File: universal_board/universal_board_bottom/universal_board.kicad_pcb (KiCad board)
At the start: 2 copper layers, 39.1 x 45.8 mm, 26 parts

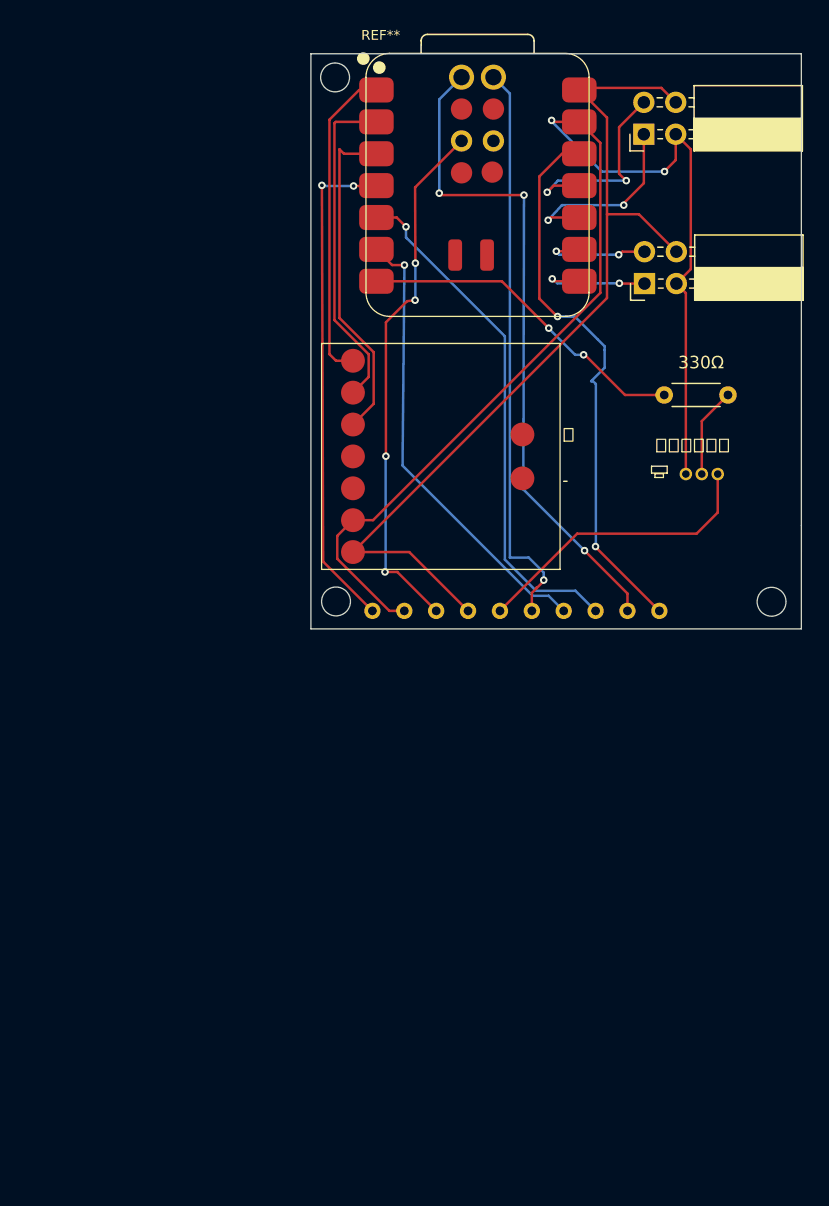
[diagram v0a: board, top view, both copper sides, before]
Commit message: OLED 0.1
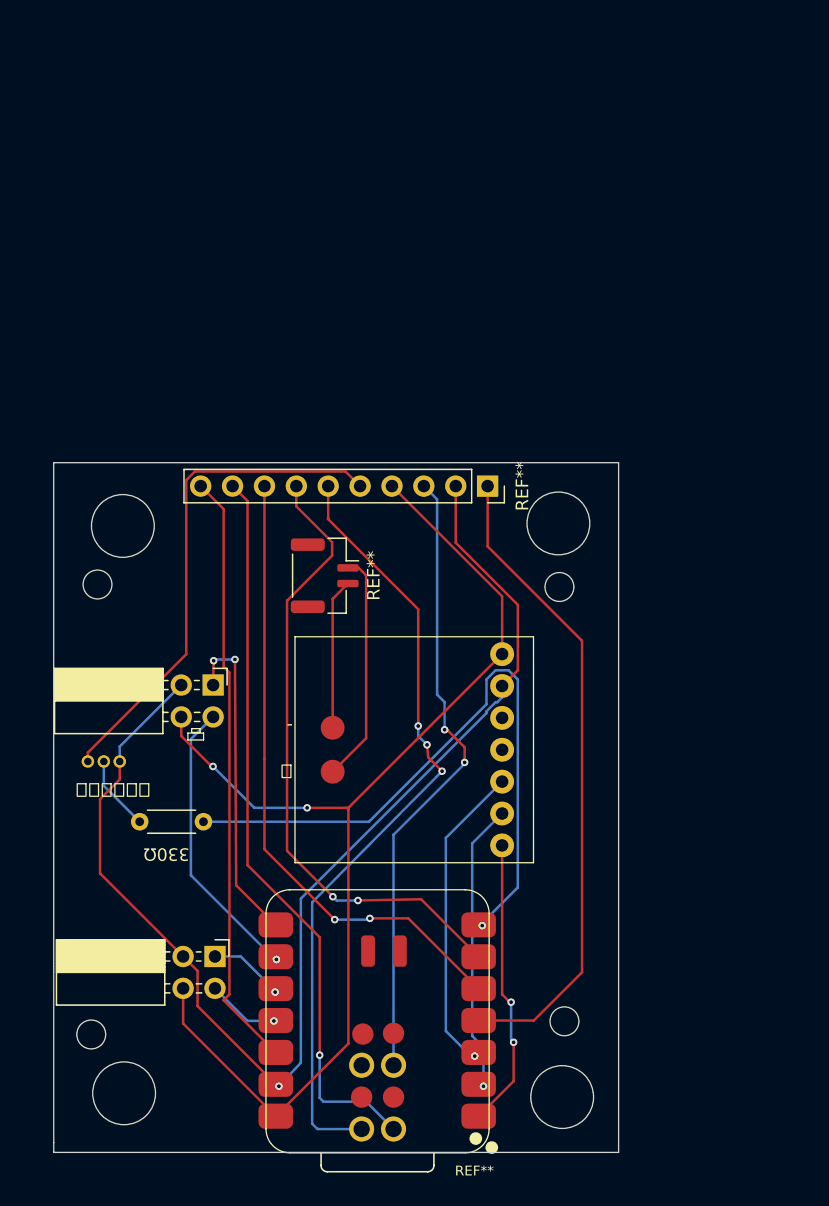
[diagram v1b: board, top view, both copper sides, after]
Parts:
- removed 19, 20, 21, 22, 23, 24, 25, 26, 27: , 
- removed the 2 at (228.2, 60.6)
- removed the 2 at (240.5, 60.4)
- removed the ? at (240.4, 60.9)
- removed the ? at (215.4, 71.8)
- removed the ? at (228.2, 65.7)
- added 2: , , F.Cu at (211.4, 81.6)
- added 2: , , F.Cu at (199.1, 81.9)
- added ?: , , F.Cu at (195.3, 83.7)
- added ?: , , F.Cu at (211.4, 76.6)
- added REF**: PinSocket_1x10_P2.54mm_Vertical, Connector_PinSocket_2.54mm:PinSocket_1x10_P2.54mm_Vertical, F.Cu at (224.6, 61.8)
- added REF**: JST_GH_SM02B-GHS-TB_1x02-1MP_P1.25mm_Horizontal, Connector_JST:JST_GH_SM02B-GHS-TB_1x02-1MP_P1.25mm_Horizontal, F.Cu at (211.6, 68.9)
- moved dadada 73.9 mm to (202.9, 99.3), turned to 0 degrees
- moved REF** 67.1 mm to (215.6, 104.4), turned to 180 degrees
- moved 9 55.2 mm to (192.7, 83.7), turned to 180 degrees
- moved 8 52.9 mm to (194.0, 83.7), turned to 180 degrees
- moved 7 50.3 mm to (199.1, 85.4), turned to -90 degrees
- moved REF** 50.0 mm to (201.9, 88.5), turned to 180 degrees
- moved dawdad 46.9 mm to (202.7, 77.7), turned to 0 degrees
- moved 6 44.6 mm to (211.4, 91.8), turned to -90 degrees
- moved 5 40.0 mm to (211.4, 89.3), turned to -90 degrees
- moved 4 35.4 mm to (211.4, 86.7), turned to -90 degrees
- moved 3 31.1 mm to (211.4, 84.2), turned to -90 degrees
- moved 1 23.2 mm to (211.4, 79.1), turned to -90 degrees
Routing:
- net 7: track 26.9 -> 52.3 mm, vias 2 -> 1
- net 5V: track 72.2 -> 92.0 mm, vias 0 -> 2
- net A_GND: track 0.00 -> 18.4 mm
- net 14: track 45.6 -> 63.2 mm, vias 1 -> 3
- net IR: track 23.7 -> 40.3 mm
- net 8: track 9.90 -> 26.3 mm
- net 6: track 36.5 -> 50.7 mm, vias 1 -> 2
- net 9: track 9.37 -> 23.2 mm, vias 2 -> 1
- net A_V: track 0.00 -> 12.0 mm
- net 4: track 40.0 -> 51.7 mm, vias 2 -> 0
- net 11: track 17.0 -> 5.87 mm, vias 2 -> 1
- net 10: track 15.9 -> 6.27 mm, vias 2 -> 1
- net 5: track 41.4 -> 50.9 mm, vias 1 -> 2
- net 15: track 42.9 -> 50.4 mm, vias 4 -> 2
- net 13: track 53.5 -> 58.5 mm, vias 3 -> 1
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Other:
- board size 39.1 x 45.8 mm -> 45 x 54.9 mm
